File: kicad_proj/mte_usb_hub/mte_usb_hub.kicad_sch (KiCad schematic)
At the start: 20 parts, among them J1 Conn_01x02_Male, J2 USB_C_Receptacle, J3 USB3_A, J4 USB3_A, J5 USB3_A, J6 USB3_A

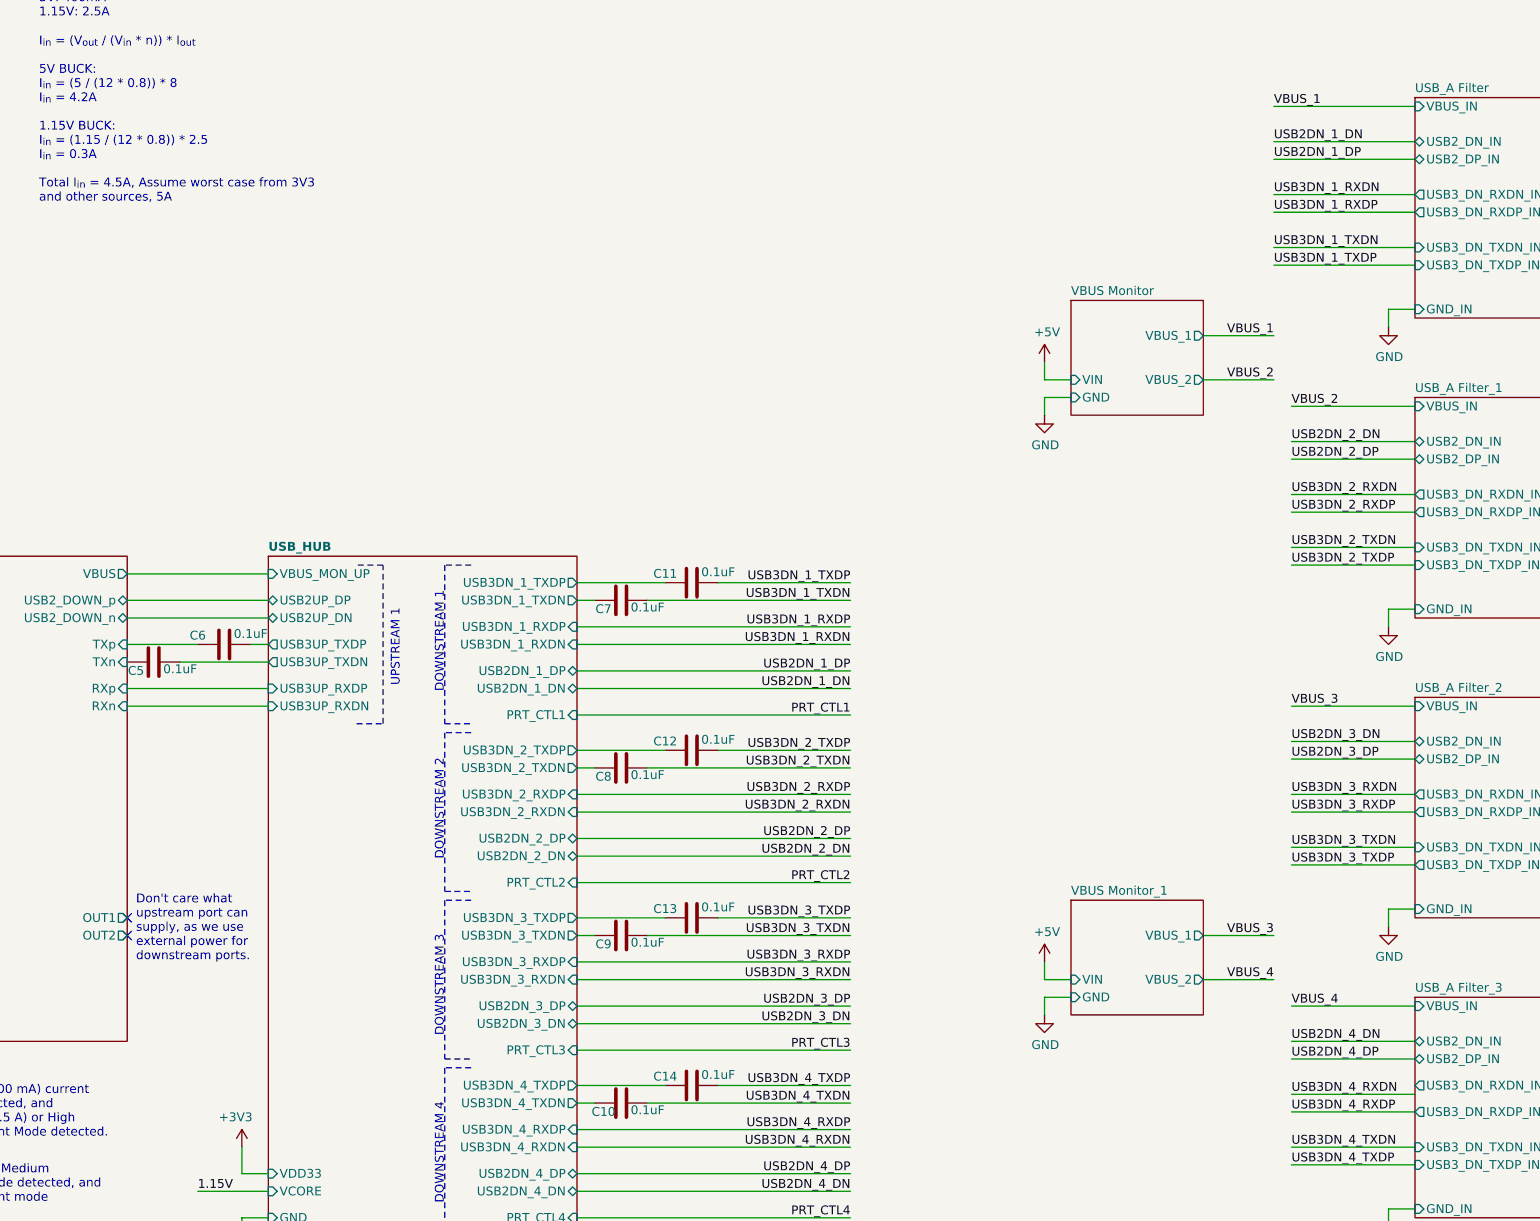
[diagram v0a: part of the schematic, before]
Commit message: Updates from the livestream
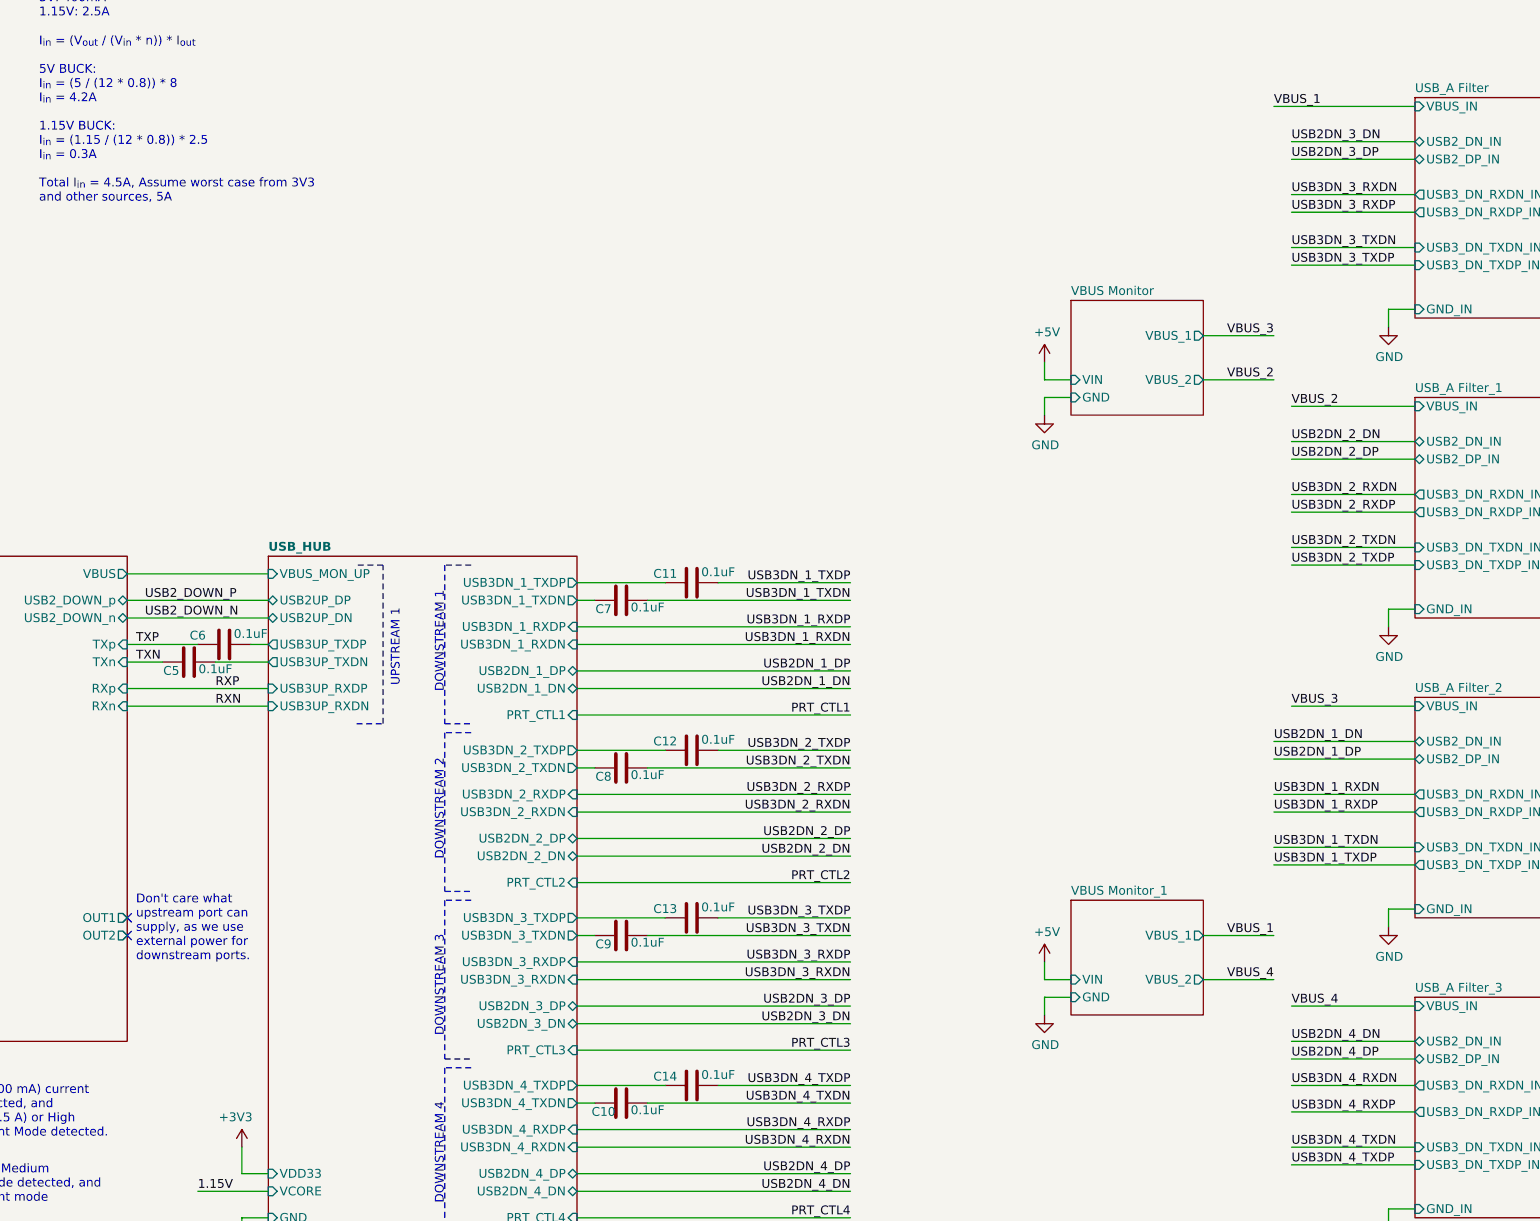
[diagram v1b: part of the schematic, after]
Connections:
- net UFP_MUX/TXn renamed TXN
- net UFP_MUX/TXp renamed TXP
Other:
- moved on the sheet: C5

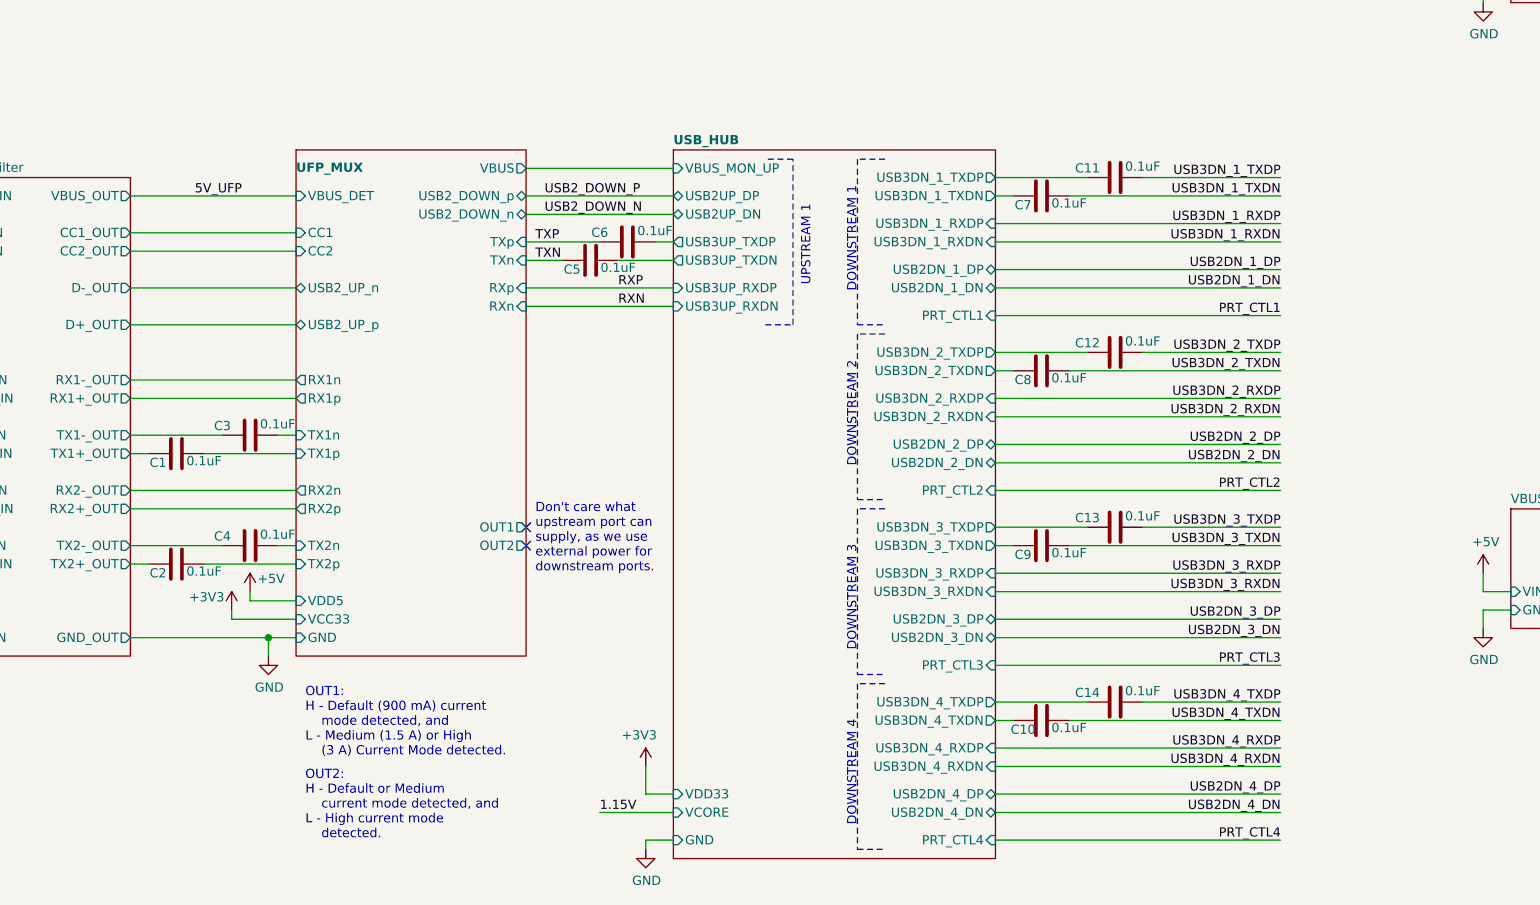
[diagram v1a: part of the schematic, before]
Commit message: Updates from the livestream
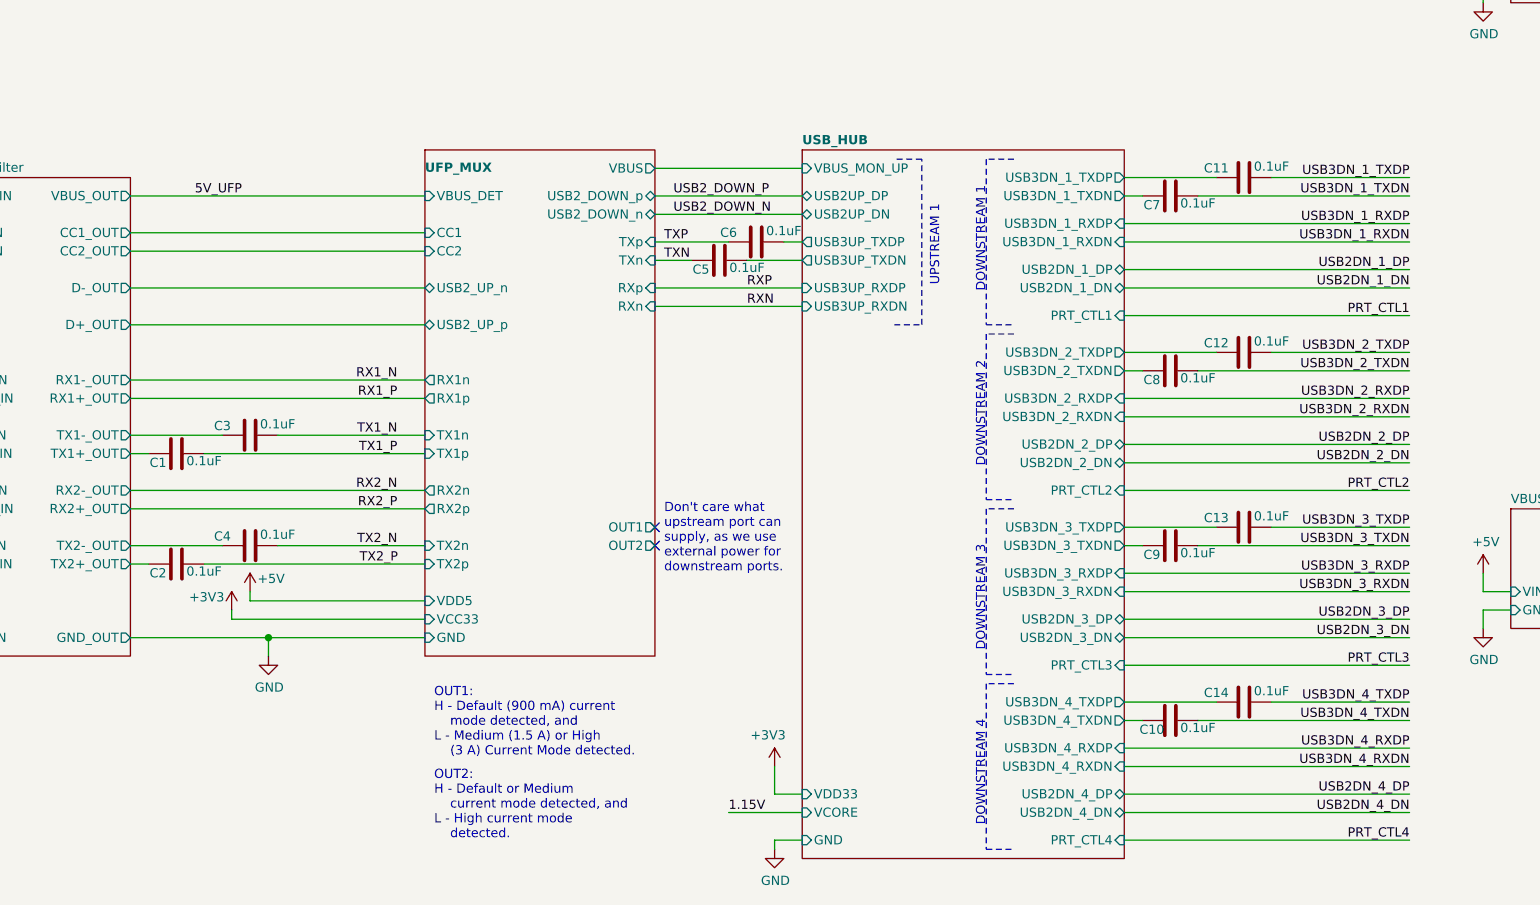
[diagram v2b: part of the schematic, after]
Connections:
- net UFP_MUX/TX1n renamed TX1_N
- net UFP_MUX/TX1p renamed TX1_P
- net UFP_MUX/TX2n renamed TX2_N
- net UFP_MUX/TX2p renamed TX2_P
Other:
- moved on the sheet: C10, C11, C12, C13, C14, C5, C6, C7, C8, C9
